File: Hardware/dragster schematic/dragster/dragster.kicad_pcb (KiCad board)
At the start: 2 copper layers, 78.9 x 75 mm, 51 parts, among them J1 Conn_01x02, J2 Conn_01x02, J3 Conn_02x07_Odd_Even, J4 Conn_01x08, J5 Conn_01x03, J6 Conn_01x02, SW2 SW_Push, U1 STM32L412KBTx, U2 MAX5033DUSA+T, U4 MAX5033DUSA+T

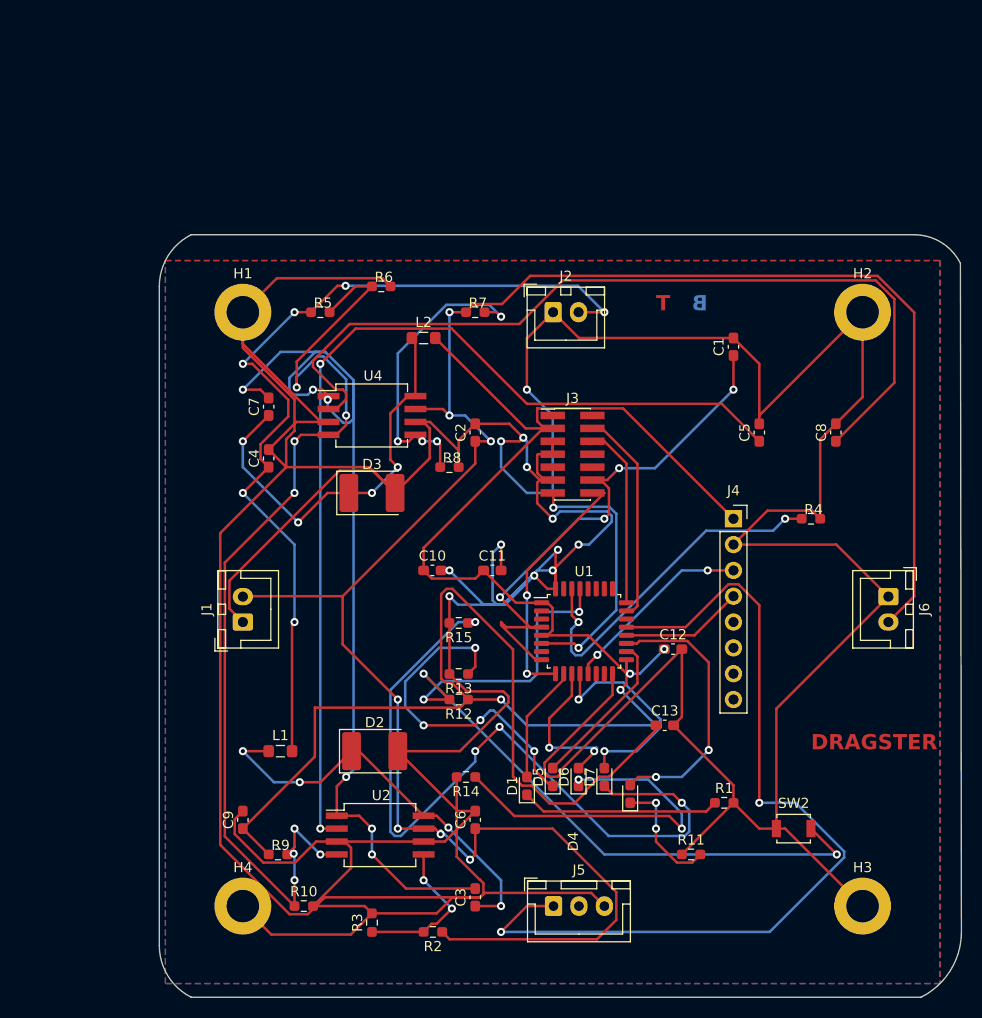
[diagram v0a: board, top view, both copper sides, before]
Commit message: Add files via upload
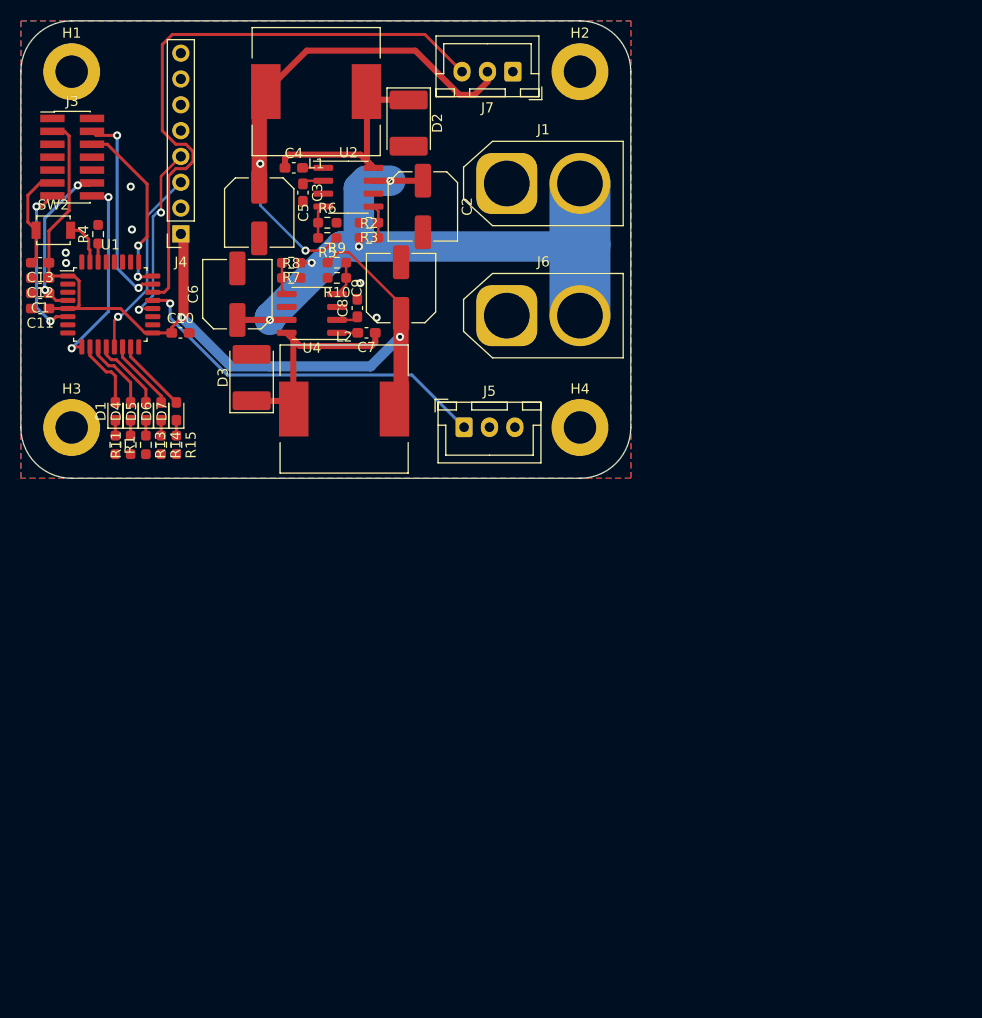
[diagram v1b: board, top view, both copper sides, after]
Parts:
- removed J2: Conn_01x02, Connector_JST:JST_XH_B2B-XH-A_1x02_P2.50mm_Vertical
- removed R12: 100k, Resistor_SMD:R_0603_1608Metric_Pad0.98x0.95mm_HandSolder
- added J7: Conn_01x03, Connector_JST:JST_XH_B3B-XH-A_1x03_P2.50mm_Vertical, F.Cu at (143.4, 50.0)
- C13: value 100n -> 1u
- C2: value 47u -> 47uF; footprint Capacitor_SMD:C_0603_1608Metric_Pad1.08x0.95mm_HandSolder -> Capacitor_SMD:C_Elec_6.3x5.4
- C3, C7: value 47uF -> 100n
- C4: value 33uF -> 100n
- C5: value 0.1u -> 33uF; footprint Capacitor_SMD:C_0603_1608Metric_Pad1.08x0.95mm_HandSolder -> Capacitor_SMD:C_Elec_6.3x5.4
- C6, C9: footprint Capacitor_SMD:C_0603_1608Metric_Pad1.08x0.95mm_HandSolder -> Capacitor_SMD:C_Elec_6.3x5.4
- C8: value 0.1u -> 100n
- J1, J6: footprint Connector_JST:JST_XH_B2B-XH-A_1x02_P2.50mm_Vertical -> Connector_AMASS:AMASS_XT60-M_1x02_P7.20mm_Vertical
- L1, L2: footprint Inductor_SMD:L_0805_2012Metric_Pad1.05x1.20mm_HandSolder -> Inductor_SMD:L_12x12mm_H6mm
- R2, R7: value R_Small -> 1M
- R3, R8: value R_Small -> 384k
- U2, U4: footprint Package_SO:SSO-8_6.8x5.9mm_P1.27mm_Clearance7mm -> Package_SO:SOIC-8_3.9x4.9mm_P1.27mm
- moved SW2 93.6 mm to (98.2, 65.6)
- moved H3 90.9 mm to (100.0, 85.0)
- moved C13 76.5 mm to (96.9, 68.8), turned to 180 degrees
- moved R4 75.5 mm to (102.6, 66.0), turned to 90 degrees
- moved C12 72.2 mm to (96.9, 70.3), turned to 180 degrees
- moved C3 71.4 mm to (122.8, 61.9), turned to -90 degrees
- moved R1 69.5 mm to (104.3, 86.7), turned to -90 degrees
- moved R3 68.8 mm to (129.2, 64.9), turned to 180 degrees
- moved R2 68.6 mm to (129.2, 66.3), turned to 0 degrees
- moved C1 68.4 mm to (96.9, 71.8), turned to 180 degrees
- moved R11 68.3 mm to (105.8, 86.7), turned to 90 degrees
- moved L1 65.0 mm to (124.0, 52.0), turned to 180 degrees
- moved U2 63.8 mm to (127.2, 61.4)
- moved D4 61.9 mm to (105.8, 83.4)
- moved R10 61.9 mm to (126.1, 70.3), turned to 180 degrees
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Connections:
- net Vin_regulateur renamed +12V
- C3 pad 1: LX -> Net-(U2-VD)
- C3 pad 2: BST -> GND
- C4 pad 1: +7.5V -> Net-(D2-K)
- C4 pad 2: GND -> BST
- C5 pad 1: VD -> +7.5V
- C7 pad 2: BST -> BST1
- D2 pad 1: LX -> Net-(D2-K)
- L1 pad 1: LX -> Net-(D2-K)
- R10 pad 1: FB -> FB1
- R5 pad 2: FB -> FB2
- R6 pad 1: FB -> FB2
- R9 pad 2: FB -> FB1
- U1 pad 11: Led_Status3 -> Led_Status1
- U1 pad 12: Led_Status4 -> Led_Status
- U1 pad 14: unconnected-(U1-PB0-Pad14) -> Led_Status3
- U1 pad 15: unconnected-(U1-PB1-Pad15) -> Led_Status4
- U1 pad 18: Led_Status -> unconnected-(U1-PA8-Pad18)
- U1 pad 19: Led_Status1 -> unconnected-(U1-PA9-Pad19)
- U1 pad 22: unconnected-(U1-PA12-Pad22) -> DATA SVM
- U1 pad 29: Bouton_USR -> unconnected-(U1-PB6-Pad29)
- U1 pad 31: unconnected-(U1-PH3-Pad31) -> Bouton_USR
- U1 pad 8: NRST -> unconnected-(U1-PA2-Pad8)
- U2 pad 2: VD -> Net-(U2-VD)
- U2 pad 4: FB -> FB2
- U2 pad 8: LX -> Net-(D2-K)
- U4 pad 1: BST -> BST1
- U4 pad 4: FB -> FB1
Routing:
- net GND: track 633.2 -> 10.1 mm, vias 12 -> 6
- net +12V: track 205.8 -> 67.7 mm, vias 7 -> 4
- net +3.3V: track 211.8 -> 94.2 mm, vias 4 -> 2
- net FB: track 101.4 -> 0.00 mm, vias 8 -> 0
- net VD: track 96.5 -> 0.00 mm, vias 2 -> 0
- net BST: track 96.7 -> 2.04 mm, vias 6 -> 0
- net Net-(U4-VD): track 85.3 -> 2.13 mm
- net Bouton_USR: track 82.5 -> 4.43 mm, vias 4 -> 0
- net Net-(D7-K): track 76.5 -> 1.51 mm, vias 4 -> 0
- net DATA SVM: track 0.00 -> 60.5 mm
- net ESC1: track 89.0 -> 36.6 mm, vias 2 -> 1
- net LX: track 40.8 -> 0.00 mm, vias 4 -> 0
- net NRST: track 54.7 -> 15.8 mm, vias 4 -> 2
- net +7.5V: track 87.6 -> 52.7 mm, vias 6 -> 2
- net Net-(D6-K): track 36.1 -> 1.51 mm, vias 2 -> 0
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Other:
- board size 78.9 x 75 mm -> 60 x 45 mm
- board text removed: "B"
- board text removed: "DRAGSTER"
- board text removed: "T"
